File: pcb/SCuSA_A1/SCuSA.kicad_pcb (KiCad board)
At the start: 2 copper layers, 56 x 68 mm, 63 parts, among them J101 USB4135-GF-A, J102 JST_S2B-PH-K-x, J103 Binding_Post_PK4_Red, J104 Binding_Post_PK4_Black, J105 SMA_Straight_Jack_Female, J107 77311-118-02LF, J108 77311-118-02LF, Q101 DMN2041LSD, SW101 JS202011CQN, SW102 JS202011CQN, U101 MCP73832T-2ACI/OT, U102 BQ297xy, U103 TLV803EA30DBZR, U104 LM27762, U105 AD8410AWBRZ, U106 AD8655ARZ

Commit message: Preliminary BOM
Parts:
- C106: value 470nF,25V,X7R,0603 -> 1uF,16V,X7R,0603
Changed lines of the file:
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@@
         (effects (font (size 1 1) (thickness 0.15)))
     )
-    (fp_text value "470nF,25V,X7R,0603" (at 0 1.43) (layer "F.Fab")
+    (fp_text value "1uF,16V,X7R,0603" (at 0 1.43) (layer "F.Fab")
         (effects (font (size 1 1) (thickness 0.15)))
     )

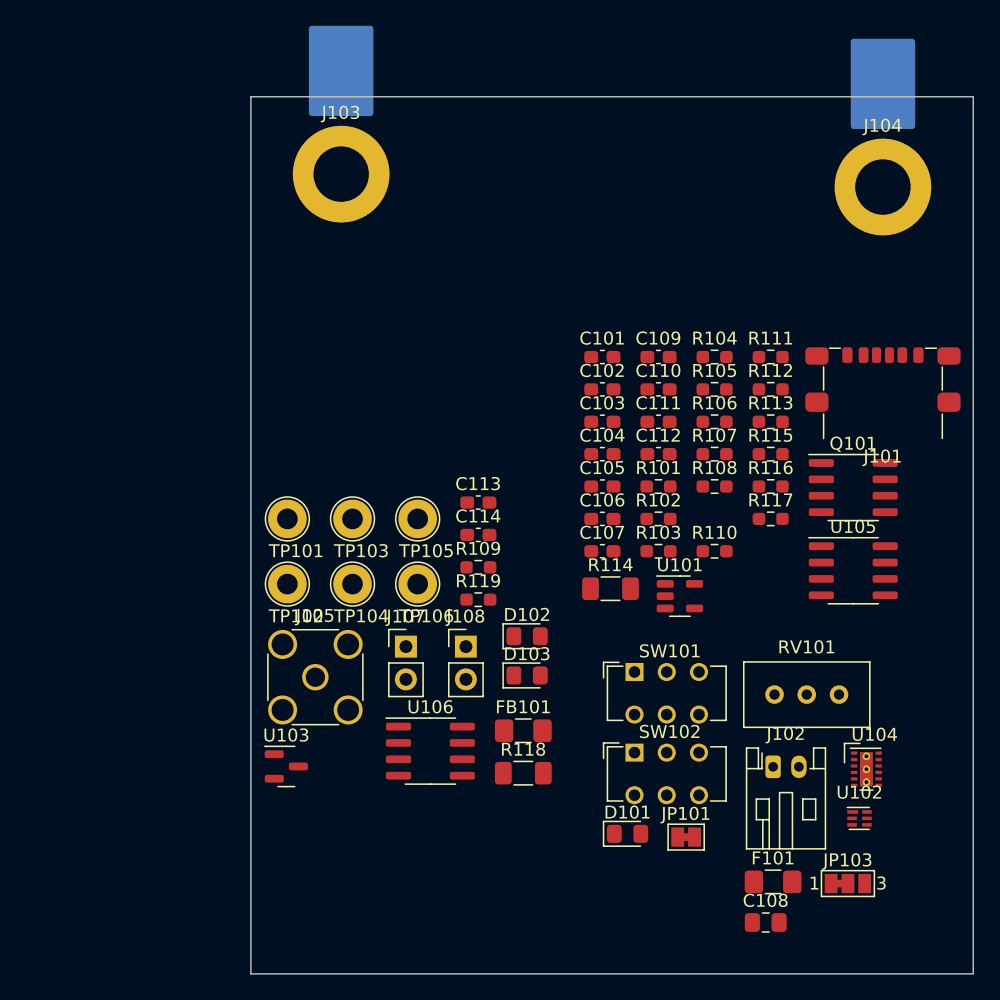
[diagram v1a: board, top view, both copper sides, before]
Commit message: Work on PCB layout
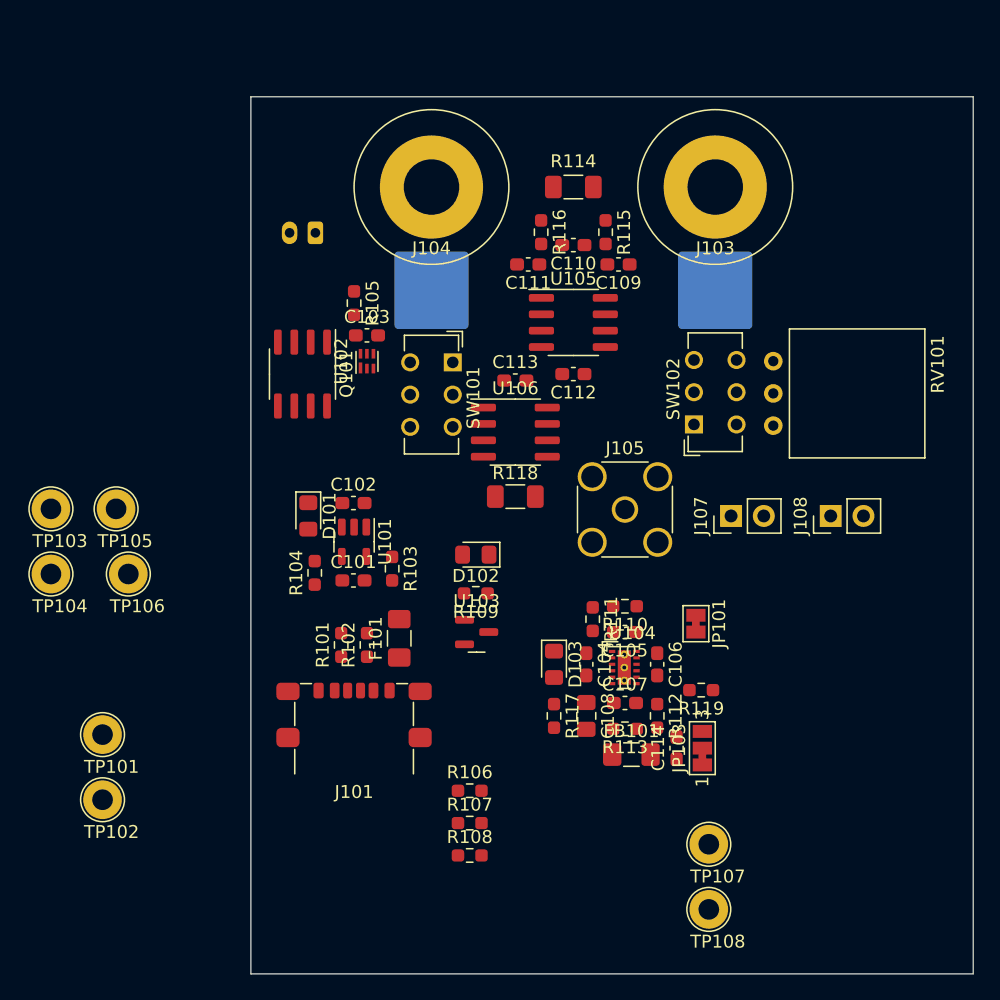
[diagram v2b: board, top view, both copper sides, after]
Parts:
- added TP107: TestPoint_5011_Black, TestPoint:TestPoint_Loop_D2.60mm_Drill1.6mm_Beaded, F.Cu at (147.5, 120.0)
- added TP108: TestPoint_5010_Red, TestPoint:TestPoint_Loop_D2.60mm_Drill1.6mm_Beaded, F.Cu at (147.5, 125.0)
- J102: moved to B.Cu
- J103: footprint Connector_User:Binding_Post_4.3mm_M4_DIN965_Pad -> Connector_User:Binding_Post_PK4_Red
- J104: footprint Connector_User:Binding_Post_4.3mm_M4_DIN965_Pad -> Connector_User:Binding_Post_PK4_Black
- J105: footprint Connector_Coaxial:SMA_Wurth_60312002114503_Vertical -> Connector_User:SMA_Vertical
- R113: value 120k,0603 -> 47k,0603
- RV101: footprint Potentionmeter_THT_User:Potentiometer_Suntan_3296W_Vertical -> Potentionmeter_THT_User:Potentiometer_Suntan_3296W_Vertical_90deg
- U102: value BQ297xy -> BQ29700DSER
- moved J102 54.5 mm to (117.0, 72.5), turned to 180 degrees
- moved U102 52.1 mm to (121.0, 82.5), turned to 90 degrees
- moved J101 48.5 mm to (120.0, 108.1)
- moved Q101 43.6 mm to (116.0, 83.5), turned to -90 degrees
- moved R104 35.2 mm to (117.0, 98.9), turned to 90 degrees
- moved J104 35.0 mm to (126.0, 69.0), turned to 180 degrees
- moved D101 34.9 mm to (116.5, 94.5), turned to -90 degrees
- moved F101 34.6 mm to (123.5, 104.0), turned to 90 degrees
- moved R107 34.3 mm to (129.0, 118.3)
- moved R106 34.3 mm to (129.0, 115.8)
- moved R108 34.3 mm to (129.0, 120.8)
- moved R114 31.3 mm to (137.0, 69.0), turned to 180 degrees
- moved J108 30.0 mm to (156.9, 94.5), turned to 90 degrees
- moved J103 29.0 mm to (148.0, 69.0), turned to 180 degrees
- moved U105 29.0 mm to (137.0, 79.5)
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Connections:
- C112 pad 2: GND -> -VOffset
